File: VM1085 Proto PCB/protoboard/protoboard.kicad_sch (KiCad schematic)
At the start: 82 parts, among them J1 Conn_01x03_Male, J10 Conn_01x03_Male, J11 Conn_01x03_Male, J12 Conn_01x03_Male, J13 Conn_01x03_Male, J14 Conn_01x03_Male, J15 Conn_01x03_Male, J16 Conn_01x03_Male, J17 Conn_01x03_Male, J2 Conn_01x08_Female, J3 Conn_01x03_Male, J4 Conn_01x03_Male, J5 Conn_01x03_Male, J6 Conn_01x03_Male, J7 Conn_01x03_Male, J8 Conn_01x03_Male, J9 Conn_01x03_Male, U1 TMUX1134, U10 OPA2145, U2 TMUX1134, U3 TMUX1134, U4 TMUX1134, U5 OPA2145, U6 AD8065, U7 SMD_1.27MM_PROTO_AREA, U8 LT1715, U9 ADG1401

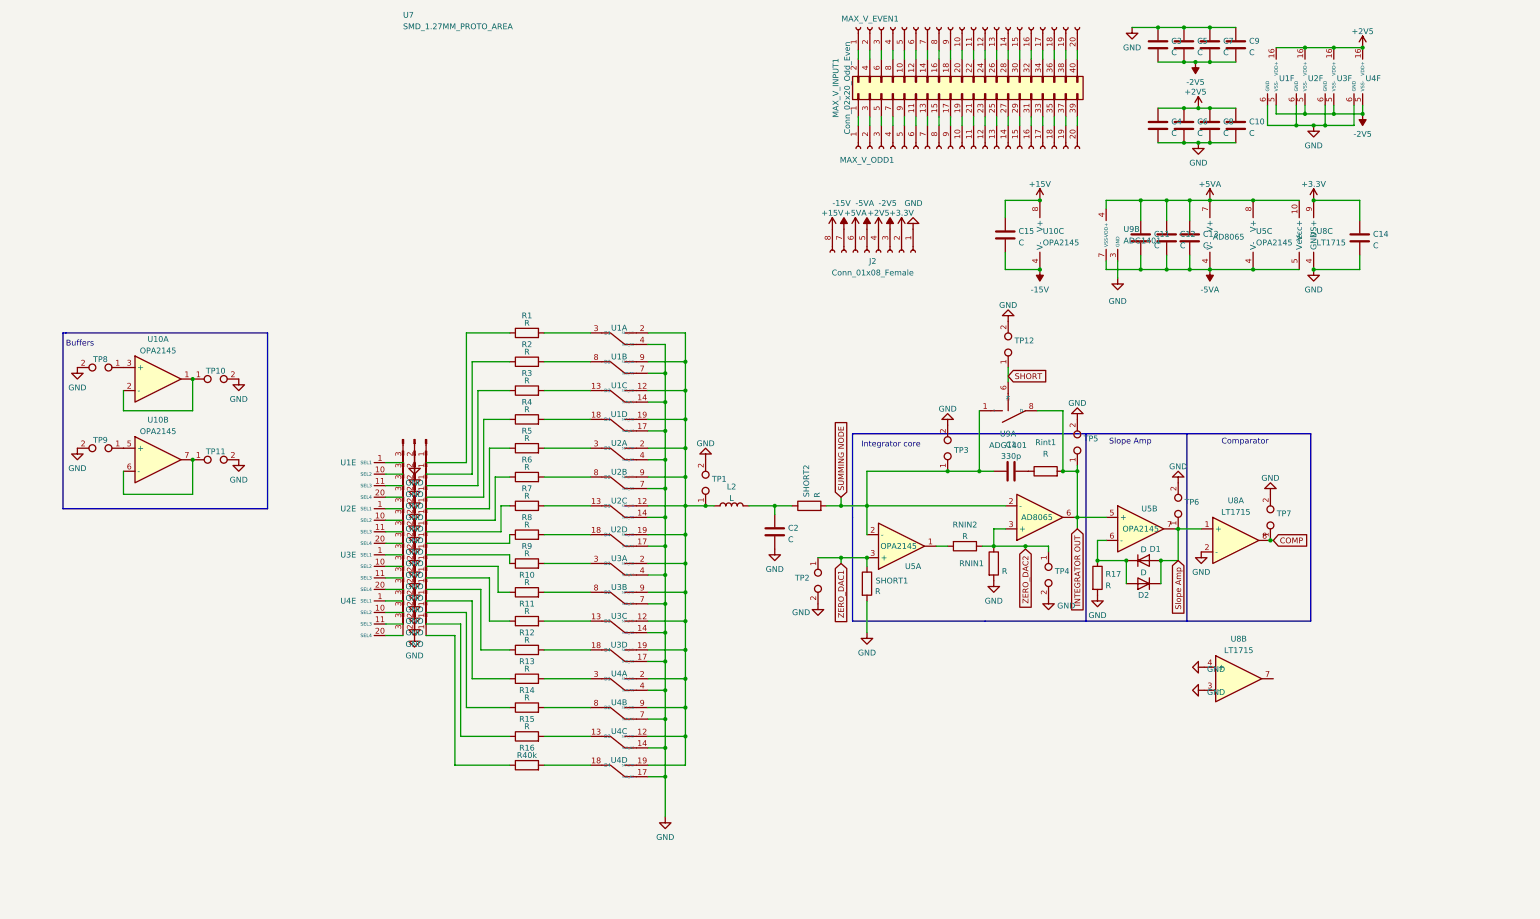
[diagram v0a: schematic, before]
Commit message: rebase save
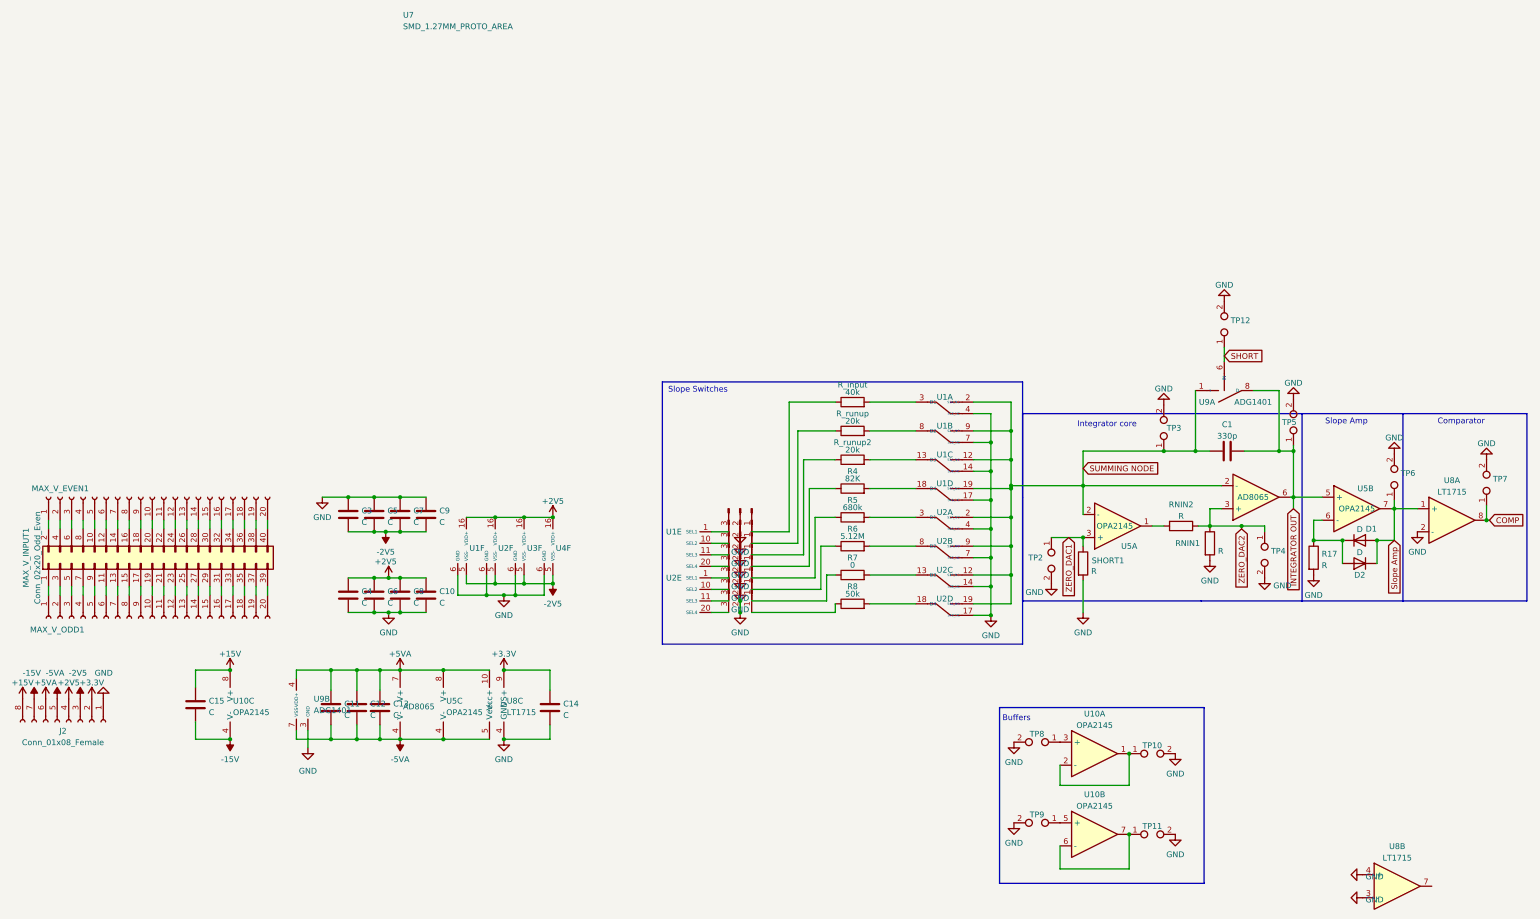
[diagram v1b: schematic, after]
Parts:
- removed C2: C, Capacitor_SMD:C_0603_1608Metric_Pad1.08x0.95mm_HandSolder, symbol Device:C
- removed J10, J11, J12, J13, J14, J15, J16, J17: Conn_01x03_Male, Connector_PinHeader_2.54mm:PinHeader_1x03_P2.54mm_Vertical, symbol Connector:Conn_01x03_Male
- removed L2: L, Capacitor_SMD:C_0805_2012Metric_Pad1.18x1.45mm_HandSolder, symbol Device:L
- removed R10, R11, R12, R13, R14, R15, R9: R, VM1085:Resistor_multipad, symbol Device:R
- removed R16: R40k, VM1085:Resistor_multipad, symbol Device:R
- removed Rint1, SHORT2: R, Resistor_SMD:R_0805_2012Metric_Pad1.20x1.40mm_HandSolder, symbol Device:R
- removed TP1: TestPoint_2Pole, Connector_PinHeader_2.54mm:PinHeader_1x02_P2.54mm_Vertical, symbol Connector:TestPoint_2Pole
- removed unit 3 of U3
- removed unit 2 of U3
- removed unit 5 of U3
- removed unit 1 of U3
- removed unit 4 of U3
- removed unit 5 of U4
- removed unit 1 of U4
- removed unit 3 of U4
- removed unit 2 of U4
- removed unit 4 of U4
- R4: value R -> 82K
- R5: value R -> 680k
- R6: value R -> 5.12M
- R7: value R -> 0
- R8: value R -> 50k
- R_input: renamed from R1; value R -> 40k
- R_runup: renamed from R2; value R -> 20k
- R_runup2: renamed from R3; value R -> 20k
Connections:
- net INTEGRATOR OUT: now also C1.2
- net SUMMING NODE: now also U1.12 (S3A_NO), U1.19 (S4A_NO), U1.2 (S1A_NO), U1.9 (S2A_NO), U2.12 (S3A_NO), U2.19 (S4A_NO), U2.2 (S1A_NO), U2.9 (S2A_NO)
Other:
- note added: "Slope Switches"
- moved on the sheet: C1, C10, C11, C12, C13, C14, C15, C3, C4, C5, C6, C7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
